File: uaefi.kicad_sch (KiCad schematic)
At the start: 66 parts, among them J1 Conn_02x02_Odd_Even, J1 USB_B_Mini, J1 USB_C, J10 5569-16A2, J11 Conn_02x02_Odd_Even, J12 Conn_02x02_Odd_Even, J13 Conn_02x02_Odd_Even, J14 Conn_02x02_Odd_Even, J15 Conn_02x02_Odd_Even, J16 Conn_02x02_Odd_Even, J17 Conn_01x06, J17 Conn_02x02_Odd_Even, J18 Conn_02x02_Odd_Even, J19 Conn_02x02_Odd_Even, J2 5569-20A2, J20 Conn_02x02_Odd_Even, J21 Conn_02x02_Odd_Even, J22 Conn_02x02_Odd_Even, J24 Conn_02x02_Odd_Even, J3 5569-06A2, J4 5569-08A2, J5 5569-18A2, J5 Conn_01x05_Male, M1 Module-power_12and5V-0.2, M3 Module-knock-0.2, M3 Module-vr-discrete-0.4, M4 Module-vr-max9924-0.1, M5 Module-wbo-0.5, M6 Module:mega-mcu100/0.3, M7 Module-can-0.1, P1 Pad, P2 Pad, P3 Pad, P4 Pad, P7 Pad, P8 Pad, U4 JDY-33

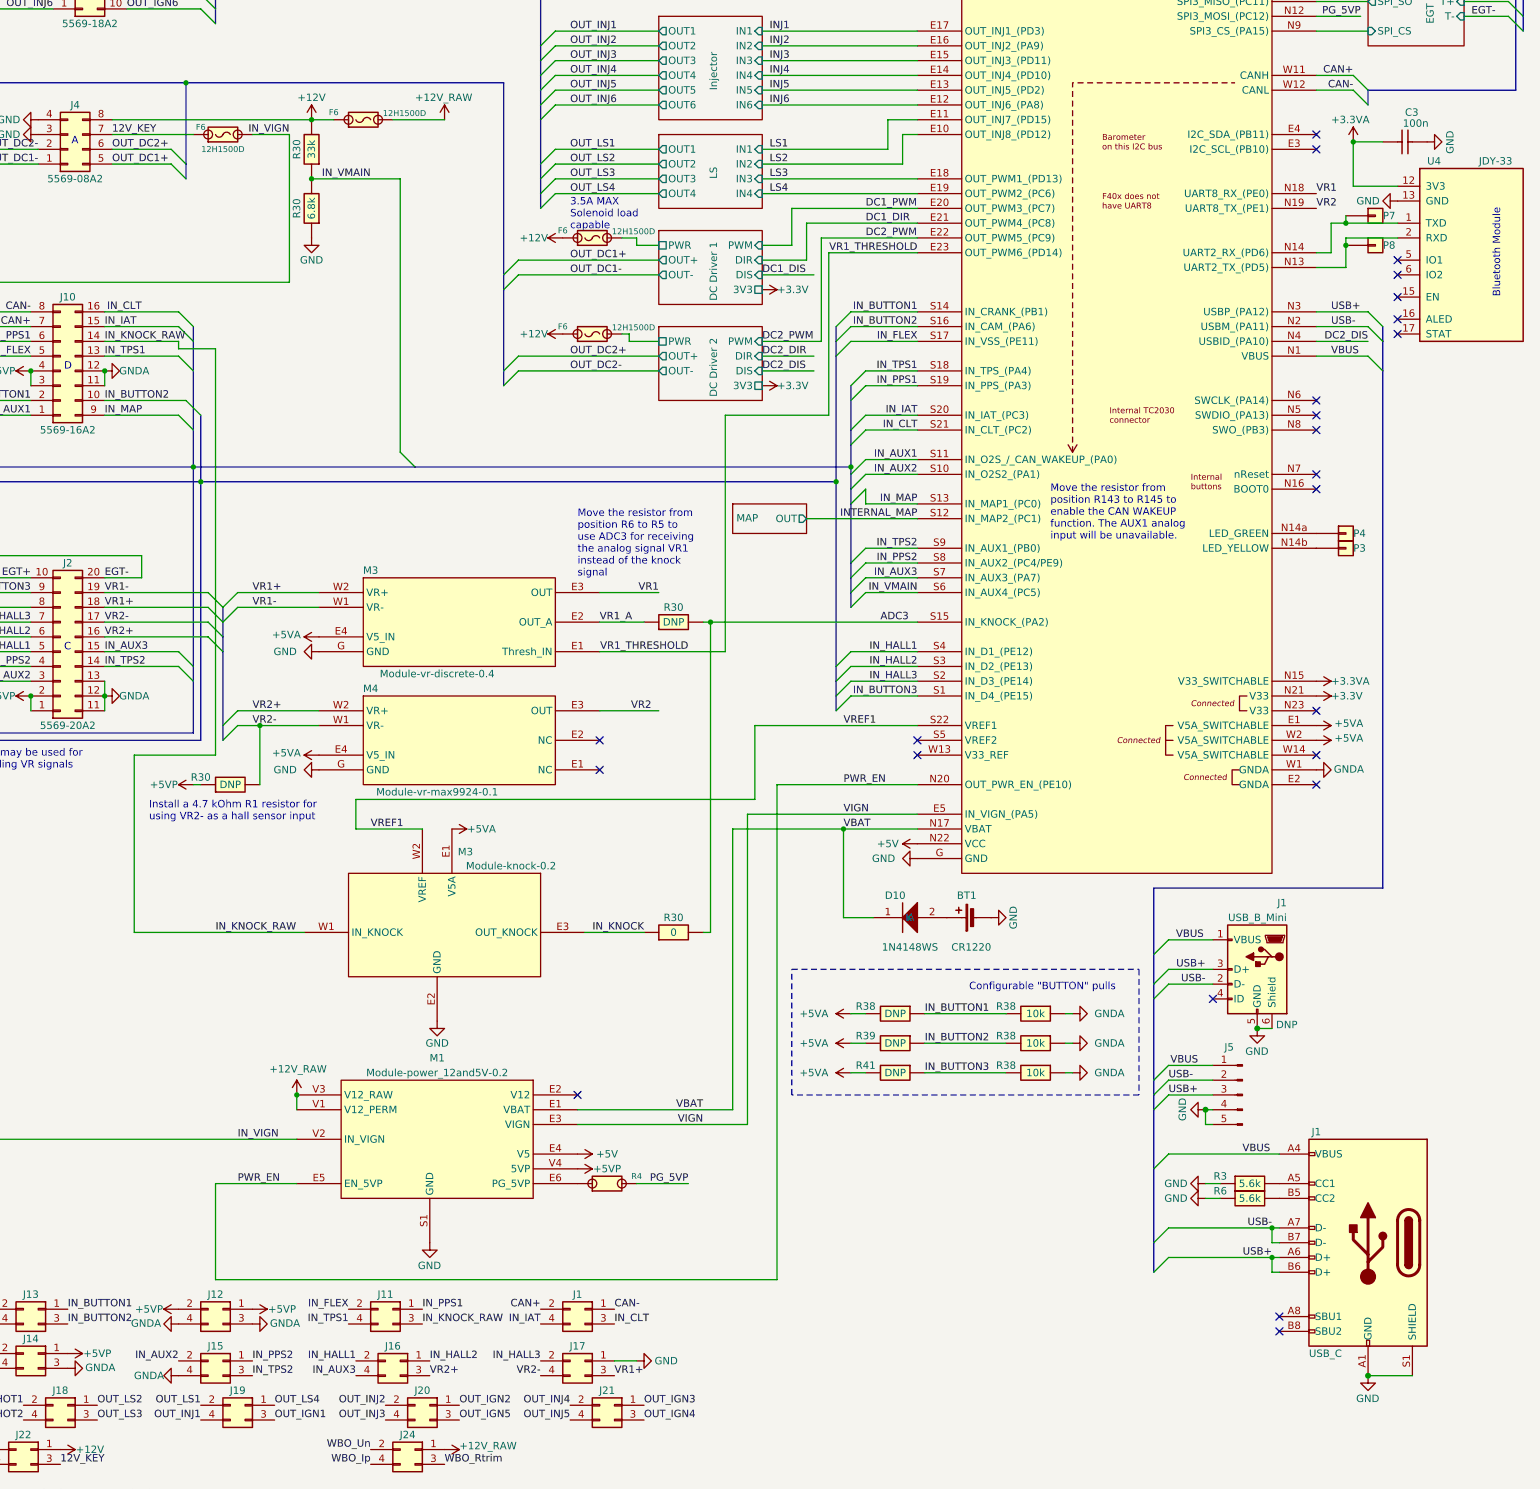
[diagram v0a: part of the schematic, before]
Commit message: Rev C
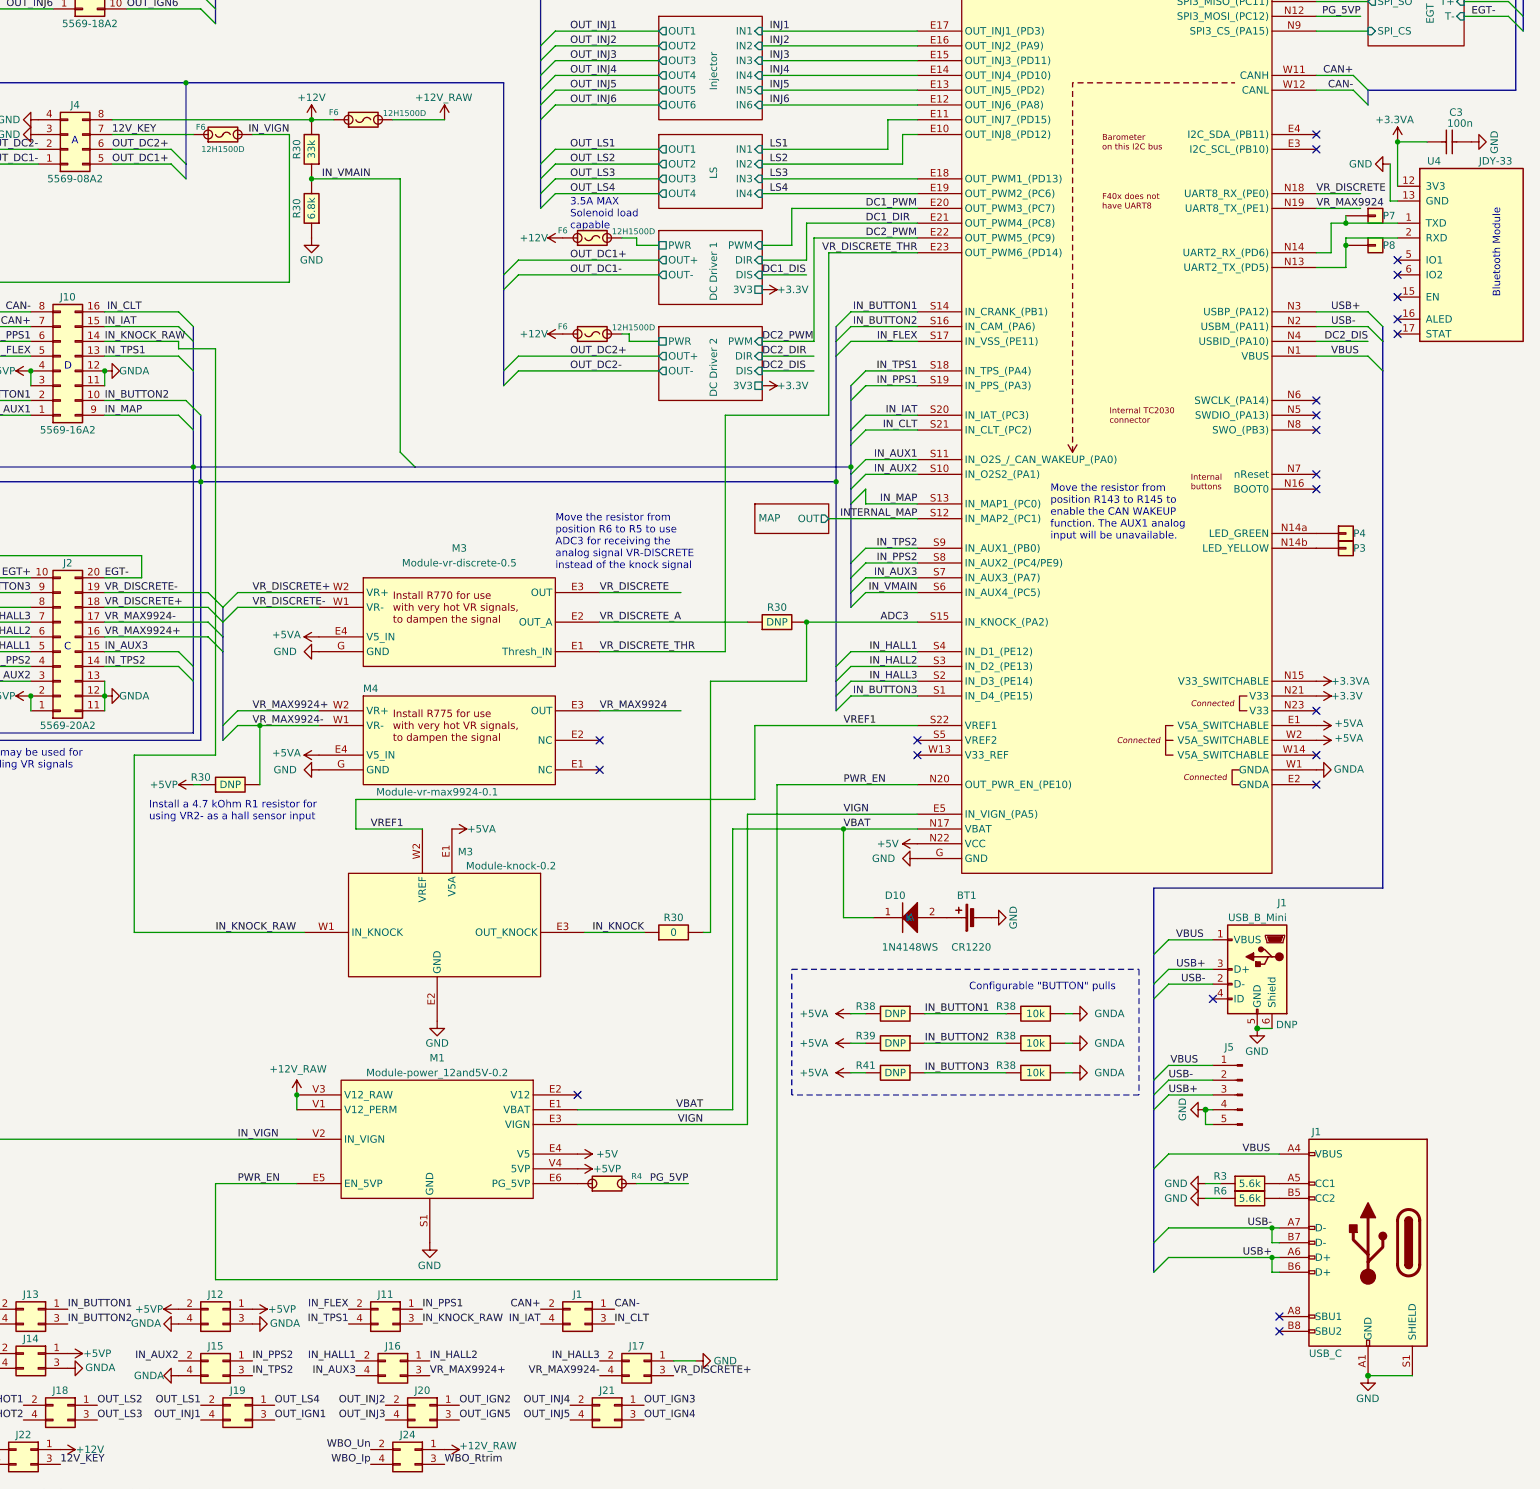
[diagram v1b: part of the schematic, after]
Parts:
- removed M3: Module-vr-discrete-0.4, hellen-one-vr-discrete-0.4:vr-discrete, symbol hellen-one-vr-discrete-0.4:Module-vr-discrete-0.4
- added M3: Module-vr-discrete-0.5, hellen-one-vr-discrete-0.5:vr-discrete, symbol hellen-one-vr-discrete-0.5:Module-vr-discrete-0.5
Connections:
- net +5VA: now also M3.E4 (V5_IN)
- net GND: now also M3.G (GND)
- net VR1 renamed VR_DISCRETE
- net VR_DISCRETE: now also M3.E3 (OUT)
- net VR1+ renamed VR_DISCRETE+
- net VR_DISCRETE+: now also M3.W2 (VR+)
- net VR1- renamed VR_DISCRETE-
- net VR_DISCRETE-: now also M3.W1 (VR-)
- net VR1_A renamed VR_DISCRETE_A
- net VR_DISCRETE_A: now also M3.E2 (OUT_A)
- net VR1_THRESHOLD renamed VR_DISCRETE_THR
- net VR_DISCRETE_THR: now also M3.E1 (Thresh_IN)
- net VR2 renamed VR_MAX9924
- net VR2+ renamed VR_MAX9924+
- net VR2- renamed VR_MAX9924-
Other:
- note added: "Move the resistor from position R6 to R5 to use ADC3 for receiving the analog signal VR-DISCRETE instead of the knock signal"
- note removed: "Move the resistor from position R6 to R5 to use ADC3 for receiving the analog signal VR1 instead of the knock signal"
- moved on the sheet: C3, J17, R30
